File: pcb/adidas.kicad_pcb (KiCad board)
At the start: 2 copper layers, 152.7 x 107.2 mm, 34 parts, among them J1 ISP Header, J2 Shitty Add-on, J4 Battery, U1 MPU-6050, U2 ATTINY841-SSU

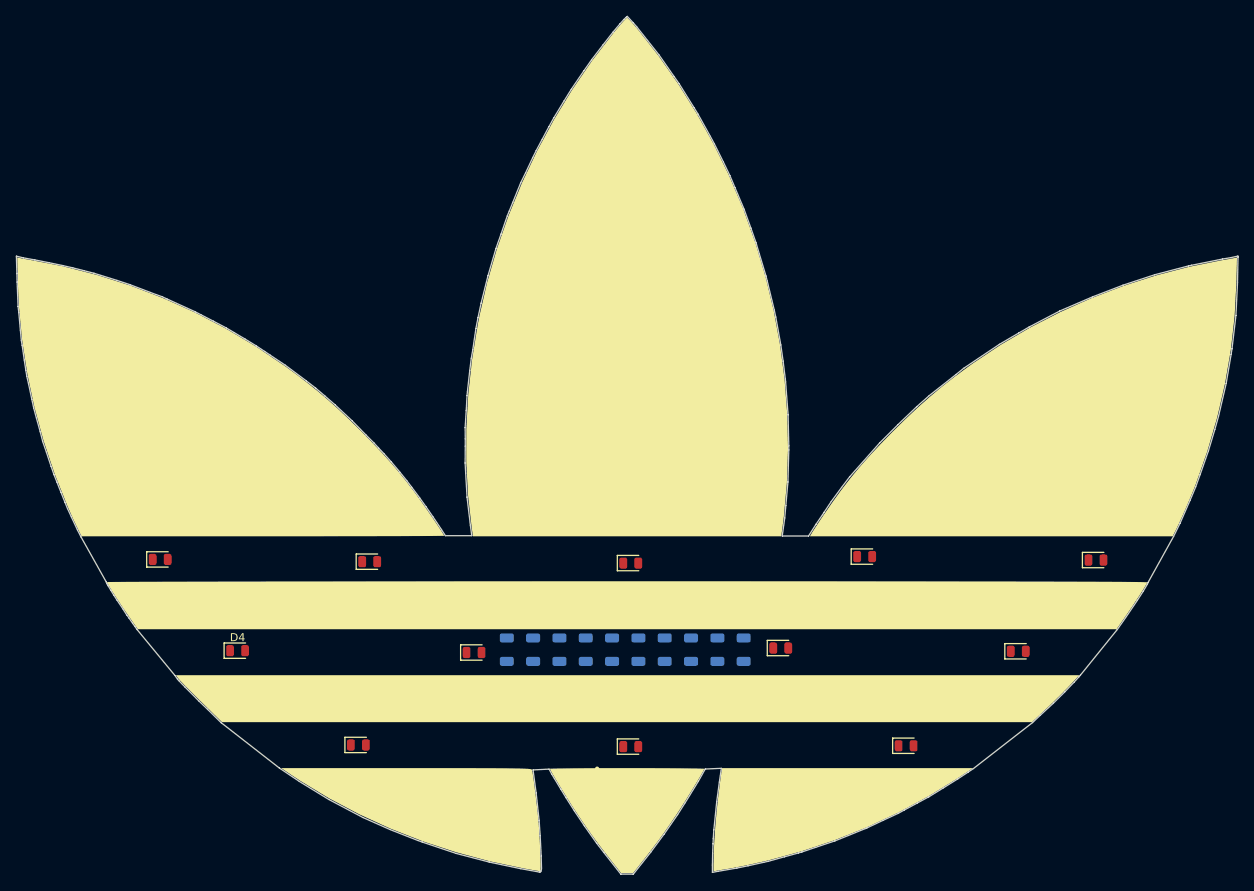
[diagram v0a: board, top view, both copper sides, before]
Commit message: RUN DRC
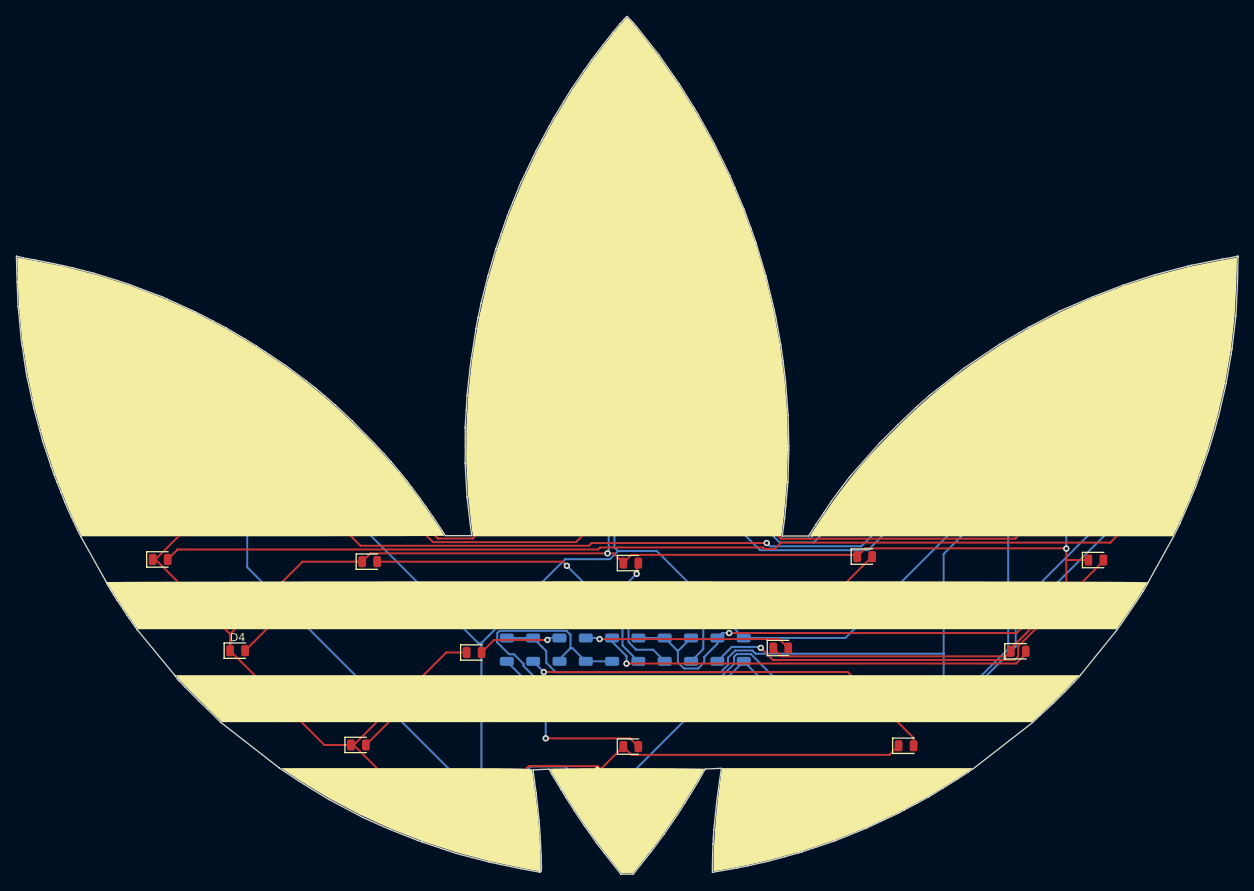
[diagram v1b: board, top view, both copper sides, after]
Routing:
- net GND: track 0.00 -> 367.1 mm, vias 0 -> 2
- net /7(SDA): track 0.00 -> 189.3 mm
- net /4(RST): track 0.00 -> 169.9 mm
- net /9(SCL): track 0.00 -> 167.8 mm, vias 0 -> 2
- net VCC: track 0.00 -> 149.7 mm
- net /3(LED Mid Row): track 0.00 -> 127.5 mm
- net Net-(D8-Pad2): track 0.00 -> 124.8 mm, vias 0 -> 1
- net Net-(J1-Pin_1): track 0.00 -> 121.6 mm, vias 0 -> 1
- net /2(LED Bottom Row): track 0.00 -> 101.6 mm
- net Net-(D4-Pad2): track 0.00 -> 100.2 mm, vias 0 -> 1
- net /13(SAO1): track 0.00 -> 92.9 mm, vias 0 -> 1
- net /12(SAO2): track 0.00 -> 90.5 mm, vias 0 -> 2
- net /5(LED Top Row): track 0.00 -> 88.3 mm, vias 0 -> 2
- net Net-(D1-Pad2): track 0.00 -> 71.6 mm, vias 0 -> 1
- net +BATT: track 0.00 -> 59.2 mm
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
